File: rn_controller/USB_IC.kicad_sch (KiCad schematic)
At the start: 1 part, among them U1 UPD720201K8-701-BAC-A

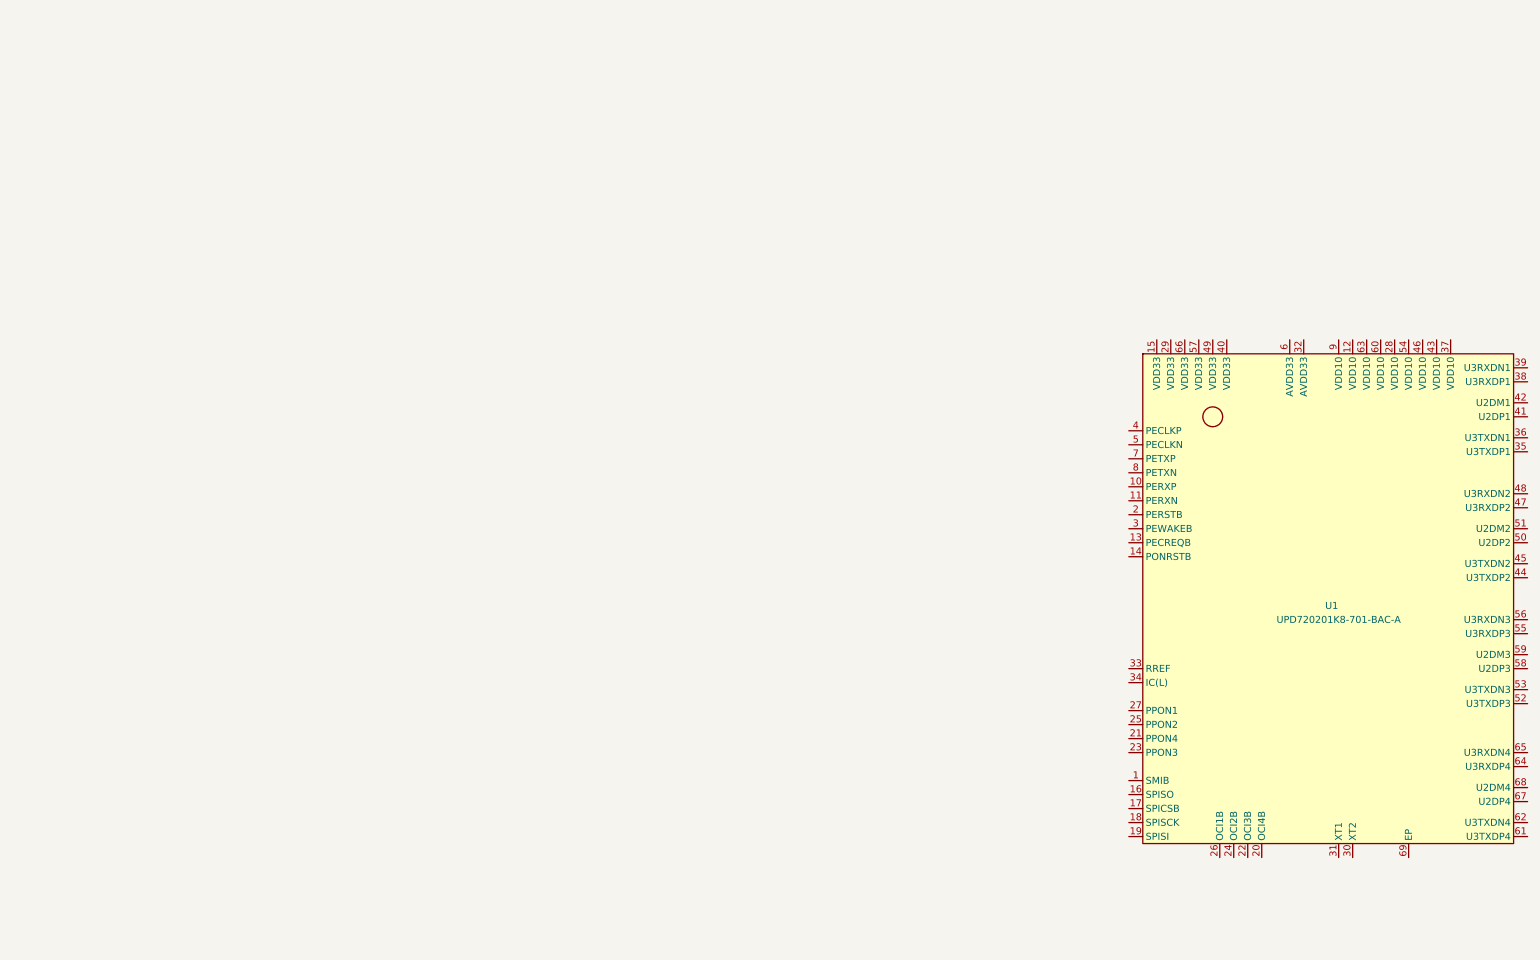
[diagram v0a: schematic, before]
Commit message: Working on part selection.
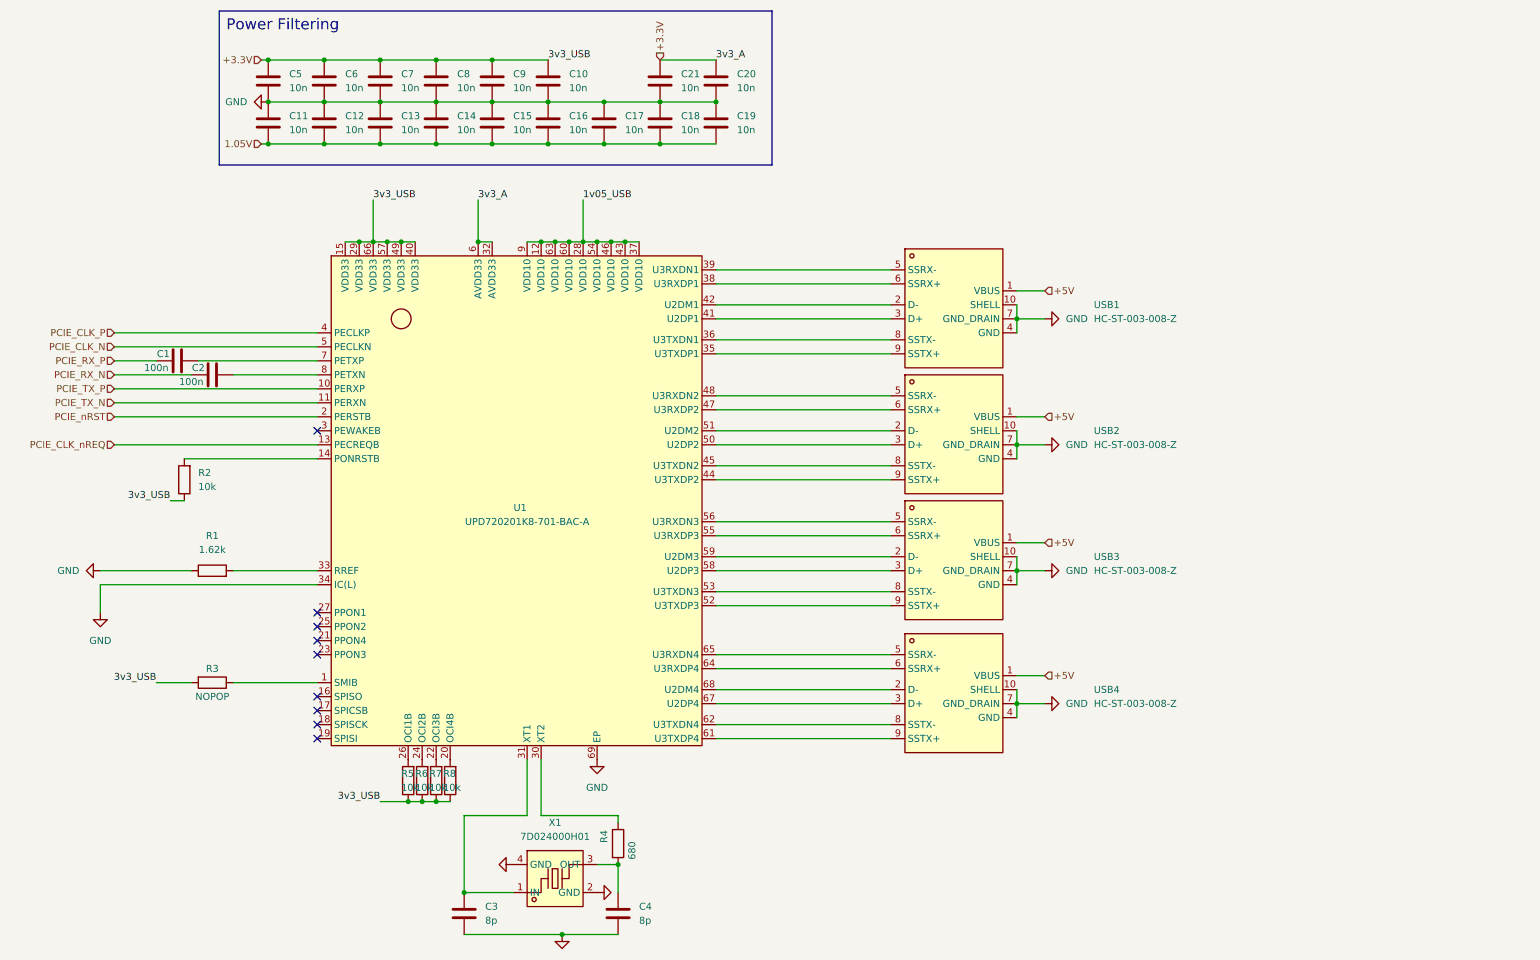
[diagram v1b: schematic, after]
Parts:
- added C1, C2: 100n, symbol Device:C
- added C10, C11, C12, C13, C14, C15, C16, C17, C18, C19, C20, C21, C5, C6, C7, C8, C9: 10n, symbol Device:C
- added C3, C4: 8p, symbol Device:C
- added R1: 1.62k, Resistor_SMD:R_0402_1005Metric, symbol Device:R
- added R2, R5, R6, R7, R8: 10k, Resistor_SMD:R_0402_1005Metric, symbol Device:R
- added R3: NOPOP, Resistor_SMD:R_0402_1005Metric, symbol Device:R
- added R4: 680, Resistor_SMD:R_0402_1005Metric, symbol Device:R
- added USB1, USB2, USB3, USB4: HC-ST-003-008-Z, NEW:USB-3.0-A-SMD_ST-003-008-J, symbol NEW:HC-ST-003-008-Z
- added X1: 7D024000H01, NEW:CRYSTAL-SMD_4P-L2.0-W1.6-BL, symbol NEW:7D024000H01
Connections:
- net at U1.1 (SMIB): now also R3.1
- net PCIE_TX_P: now reaches U1.10 (PERXP)
- net PCIE_TX_N: now reaches U1.11 (PERXN)
- net 1v05_USB: now reaches U1.12 (VDD10)
- net 1v05_USB: now also U1.28 (VDD10), U1.37 (VDD10), U1.43 (VDD10), U1.46 (VDD10), U1.54 (VDD10), U1.60 (VDD10), U1.63 (VDD10), U1.9 (VDD10)
- net PCIE_CLK_nREQ: now reaches U1.13 (PECREQB)
- net at U1.14 (PONRSTB): now also R2.2
- net +3.3V: now reaches U1.15 (VDD33)
- net +3.3V: now also U1.29 (VDD33), U1.32 (AVDD33), U1.40 (VDD33), U1.49 (VDD33), U1.57 (VDD33), U1.6 (AVDD33), U1.66 (VDD33), C10.1, C20.1, C21.1, C5.1, C6.1, C7.1, C8.1, C9.1, R2.1, R3.2, R5.1, R6.1, R7.1, R8.1
- net PCIE_nRST: now reaches U1.2 (PERSTB)
- net at U1.20 (OCI4B): now also R8.2
- net at U1.22 (OCI3B): now also R7.2
- net at U1.24 (OCI2B): now also R6.2
- net at U1.26 (OCI1B): now also R5.2
- net at U1.30 (XT2): now also R4.1
- net at U1.31 (XT1): now also C3.1, X1.1 (IN)
- net at U1.33 (RREF): now also R1.2
- net GND: now reaches U1.34 (IC(L))
- net GND: now also U1.69 (EP), C10.2, C11.1, C12.1, C13.1, C14.1, C15.1, C16.1, C17.1, C18.1, C19.1, C20.2, C21.2, C3.2, C4.2, C5.2, C6.2, C7.2, C8.2, C9.2, R1.1, USB1.10 (SHELL), USB1.4 (GND), USB1.7 (GND_DRAIN), USB2.10 (SHELL), USB2.4 (GND), USB2.7 (GND_DRAIN), USB3.10 (SHELL), USB3.4 (GND), USB3.7 (GND_DRAIN), USB4.10 (SHELL), USB4.4 (GND), USB4.7 (GND_DRAIN), X1.2 (GND), X1.4 (GND)
- net at U1.35 (U3TXDP1): now also USB1.9 (SSTX+)
- net at U1.36 (U3TXDN1): now also USB1.8 (SSTX-)
- net at U1.38 (U3RXDP1): now also USB1.6 (SSRX+)
- net at U1.39 (U3RXDN1): now also USB1.5 (SSRX-)
- net PCIE_CLK_P: now reaches U1.4 (PECLKP)
- net at U1.41 (U2DP1): now also USB1.3 (D+)
- net at U1.42 (U2DM1): now also USB1.2 (D-)
- net at U1.44 (U3TXDP2): now also USB2.9 (SSTX+)
- net at U1.45 (U3TXDN2): now also USB2.8 (SSTX-)
- net at U1.47 (U3RXDP2): now also USB2.6 (SSRX+)
- net at U1.48 (U3RXDN2): now also USB2.5 (SSRX-)
- net PCIE_CLK_N: now reaches U1.5 (PECLKN)
- net at U1.50 (U2DP2): now also USB2.3 (D+)
- net at U1.51 (U2DM2): now also USB2.2 (D-)
- net at U1.52 (U3TXDP3): now also USB3.9 (SSTX+)
- net at U1.53 (U3TXDN3): now also USB3.8 (SSTX-)
- net at U1.55 (U3RXDP3): now also USB3.6 (SSRX+)
- net at U1.56 (U3RXDN3): now also USB3.5 (SSRX-)
- net at U1.58 (U2DP3): now also USB3.3 (D+)
- net at U1.59 (U2DM3): now also USB3.2 (D-)
- net at U1.61 (U3TXDP4): now also USB4.9 (SSTX+)
- net at U1.62 (U3TXDN4): now also USB4.8 (SSTX-)
- net at U1.64 (U3RXDP4): now also USB4.6 (SSRX+)
- net at U1.65 (U3RXDN4): now also USB4.5 (SSRX-)
- net at U1.67 (U2DP4): now also USB4.3 (D+)
- net at U1.68 (U2DM4): now also USB4.2 (D-)
- net at U1.7 (PETXP): now also C1.2
- net at U1.8 (PETXN): now also C2.2
- new net: C4.1, R4.2, X1.3 (OUT)
- new net +5V: USB1.1 (VBUS), USB2.1 (VBUS), USB3.1 (VBUS), USB4.1 (VBUS)
- new net 1.05V: C11.2, C12.2, C13.2, C14.2, C15.2, C16.2, C17.2, C18.2, C19.2
- new net PCIE_RX_N: C2.1
- new net PCIE_RX_P: C1.1
- no-connect marks 0 -> 9
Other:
- note added: "Power Filtering"
- moved on the sheet: U1
